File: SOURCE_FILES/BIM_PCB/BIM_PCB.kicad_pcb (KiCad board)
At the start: 4 copper layers, 58.5 x 72.5 mm, 195 parts, among them J1 Conn_02x09_Counter_Clockwise, J2 nano_sim, J3 Conn_01x06, J4 Micro_SD_Card, Q1 SSM3J328R-HXY, Q2 SSM3J328R-HXY, Q3 IRLML0100TRPBF, Q5 BSN20, Q6 BSN20, SW1 reset, U1 STM32F103C8Tx, U10 TBU-CA065-200-WH, U11 SSP3485U, U12 TBU-CA065-200-WH, U13 ATA6561-GAQW-N, U14 WAS3157B, U15 MC74HC4052A, U16 SY8089AAAC, U17 XC6206PxxxMR, U18 TBU-CA065-200-WH, U19 SSP3485U, U2 PCF8523TK, U20 TBU-CA065-200-WH, U3 A9G_MODULE, U4 TBU-CA065-200-WH, U5 SSP3485U, U6 TBU-CA065-200-WH, U7 WAS3157B, U8 W25Q32JVSS, U9 ATA6561-GAQW-N, Y1 8MHz, Y2 32.678KHz, Y3 32.678KHz

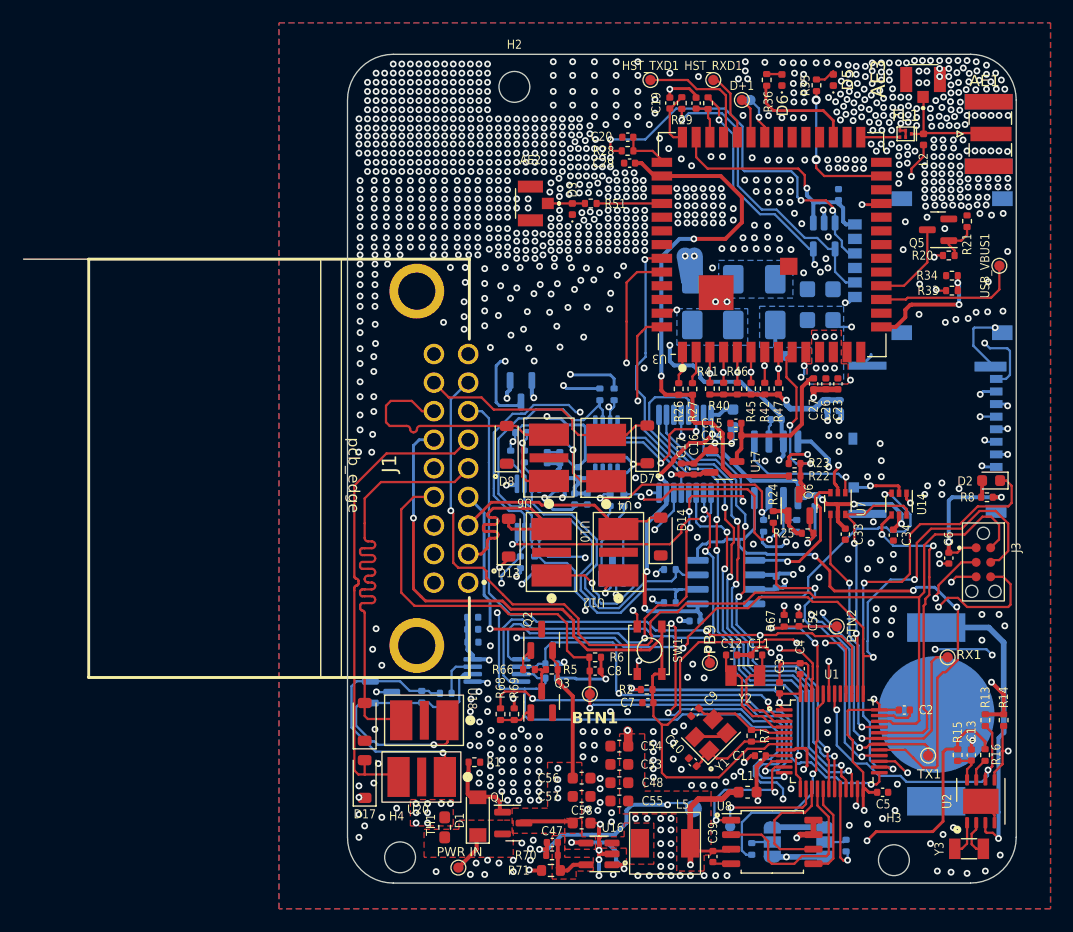
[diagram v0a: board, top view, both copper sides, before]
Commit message: all items updated
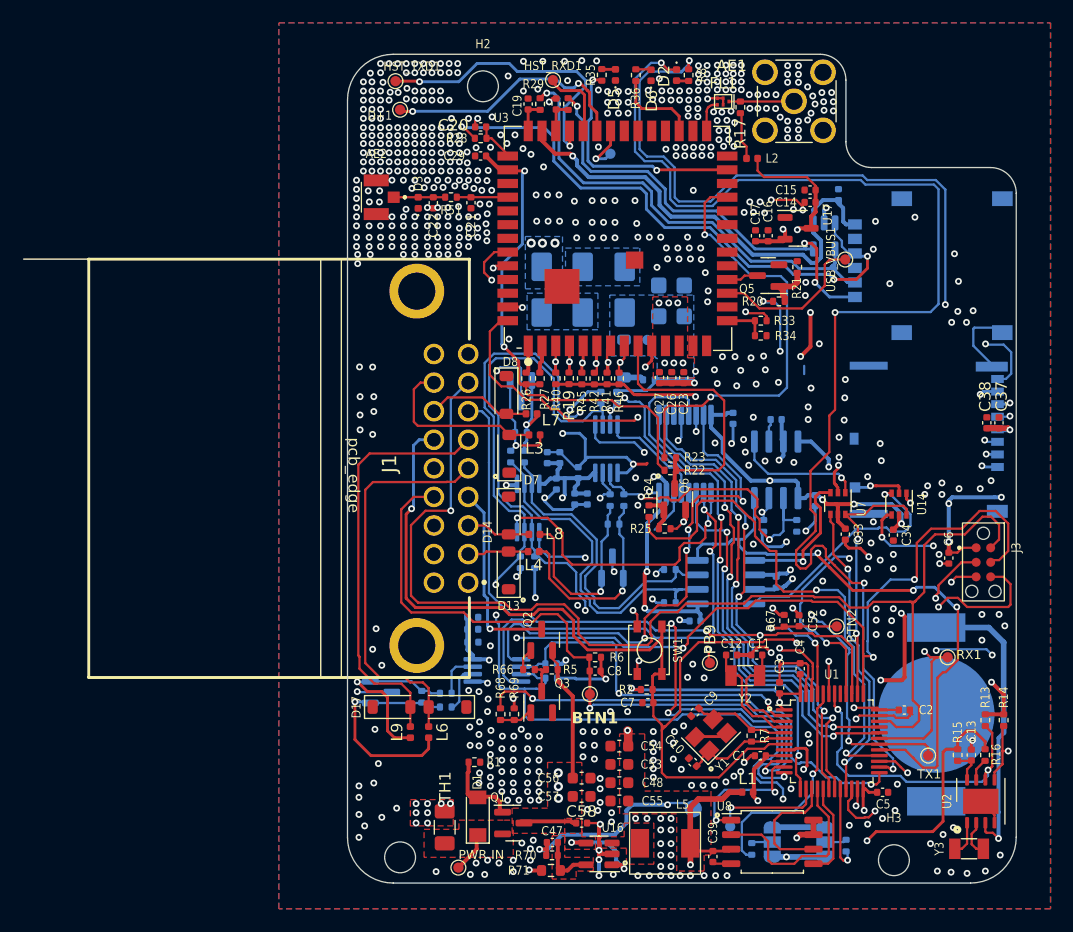
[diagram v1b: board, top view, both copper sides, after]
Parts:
- removed AE3: Antenna_Shield, greencharge-footprints:UFL_COAX_CONN23370191
- removed J4: Micro_SD_Card, MACHADA_footprints:MOLEX_503398-1892
- removed R47: 10k, Resistor_SMD:R_0402_1005Metric
- removed U10, U12, U18, U20, U4, U6: TBU-CA065-200-WH, MACHADA_footprints:TBU-CA065-200-WH
- added C37: 0.1u, Capacitor_SMD:C_0402_1005Metric, F.Cu at (93.0, 90.0)
- added C38: 1u, Capacitor_SMD:C_0402_1005Metric, F.Cu at (91.9, 90.0)
- added D19: 4.4-4.5 ZENER, Diode_SMD:D_SOD-123, B.Cu at (60.2, 84.4)
- added J7: Micro_SD_Card, MACHADA_footprints:MOLEX_503398-1892, B.Cu at (87.2, 91.5)
- added L3: ferrite bead, Inductor_SMD:L_0402_1005Metric, F.Cu at (52.4, 91.0)
- added L4: ferrite bead, Inductor_SMD:L_0402_1005Metric, F.Cu at (52.3, 101.2)
- added L6: ferrite bead, Inductor_SMD:L_0402_1005Metric, F.Cu at (43.1, 117.0)
- added L7: ferrite bead, Inductor_SMD:L_0402_1005Metric, F.Cu at (52.1, 89.2)
- added L8: ferrite bead, Inductor_SMD:L_0402_1005Metric, F.Cu at (52.4, 99.8)
- added L9: ferrite bead, Inductor_SMD:L_0402_1005Metric, F.Cu at (41.5, 117.0)
- added R17: 22R, Resistor_SMD:R_0402_1005Metric, F.Cu at (70.4, 62.4)
- added R18: 49.9R, Resistor_SMD:R_0402_1005Metric, B.Cu at (62.4, 86.2)
- added R19: 10k, Resistor_SMD:R_0402_1005Metric, F.Cu at (55.4, 86.1)
- AE1: footprint Connector_Coaxial:SMA_Samtec_SMA-J-P-X-ST-EM1_EdgeMount -> Connector_Coaxial:SMA_Molex_73251-2200_Horizontal
- C21: value 0.1u -> C_Small; moved to F.Cu
- C22: value 1u -> C_Small; moved to F.Cu
- C46, C58: footprint Capacitor_SMD:C_0603_1608Metric -> Capacitor_SMD:C_0402_1005Metric
- D10: value SS310 -> RS1K-E3/5ATSS310
- D2: footprint LED_SMD:LED_0603_1608Metric -> LED_SMD:LED_0402_1005Metric
- H4: moved to B.Cu
- L1: footprint Inductor_SMD:L_0603_1608Metric -> Inductor_SMD:L_0402_1005Metric
- Q5, Q6: value BSN20 -> IRLML0100TRPBF
- TH1: footprint Fuse:Fuse_0603_1608Metric_Pad1.05x0.95mm_HandSolder -> Fuse:Fuse_1206_3216Metric
- moved R8 45.2 mm to (65.8, 59.6), turned to -90 degrees
- moved D2 44.9 mm to (64.8, 59.6), turned to -90 degrees
- moved C22 39.7 mm to (43.5, 70.7), turned to 90 degrees
- moved C21 35.9 mm to (46.8, 70.7), turned to 90 degrees
- moved D+1 29.9 mm to (40.6, 62.6)
- moved HST_TXD1 22.3 mm to (40.2, 60.1)
- moved C15 21.4 mm to (76.5, 69.6)
- moved C16 21.4 mm to (72.8, 73.6)
- moved C17 21.4 mm to (71.7, 73.6)
- moved C14 21.4 mm to (76.5, 70.7)
- moved U17 21.4 mm to (75.4, 73.0)
- moved D5 19.1 mm to (59.4, 59.6)
- moved R35 18.8 mm to (58.2, 59.6)
- moved R34 17.5 mm to (72.2, 82.4), turned to 180 degrees
- moved AE1 17.3 mm to (75.1, 61.9), turned to -90 degrees
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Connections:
- C21 pad 1: 2V8 -> GND
- C21 pad 2: GND -> Net-(U3-GSM_RF)
- C22 pad 1: 2V8 -> GND
- C22 pad 2: GND -> Net-(AE2-A)
- L2 pad 1: Net-(AE1-A) -> Net-(L2-Pad1)
- R40 pad 2: /A9G_GSM_GPRS_MODULE/TF_CARD_CONN/SD_D2 -> /A9G_GSM_GPRS_MODULE/TF_CARD_CONN/SD_D3
- R41 pad 2: /A9G_GSM_GPRS_MODULE/TF_CARD_CONN/SD_D3 -> /A9G_GSM_GPRS_MODULE/TF_CARD_CONN/SD_CMD
- R42 pad 2: /A9G_GSM_GPRS_MODULE/TF_CARD_CONN/SD_CMD -> /A9G_GSM_GPRS_MODULE/TF_CARD_CONN/SD_D0
- R45 pad 2: /A9G_GSM_GPRS_MODULE/TF_CARD_CONN/SD_D0 -> /A9G_GSM_GPRS_MODULE/TF_CARD_CONN/SD_D1
- R46 pad 2: /A9G_GSM_GPRS_MODULE/TF_CARD_CONN/SD_D1 -> /A9G_GSM_GPRS_MODULE/TF_CARD_CONN/SD_CLK
- U1 pad 12: /A9G_GSM_GPRS_MODULE/GPS_TXD -> /A9G_GSM_GPRS_MODULE/GPS_RXD
- U1 pad 13: /A9G_GSM_GPRS_MODULE/GPS_RXD -> /A9G_GSM_GPRS_MODULE/GPS_TXD
- U1 pad 21: /STM32FC8T6_MCU/RS485_RO -> /MULTIPLEXER_SWITCH_WAS3157B-6/SIG1_IN
- U1 pad 22: /STM32FC8T6_MCU/RS485_DI -> /MULTIPLEXER_SWITCH_WAS3157B-6/SIG2_IN
- U1 pad 32: /MULTIPLEXER_SWITCH_WAS3157B-6/SIG2_IN -> /STM32FC8T6_MCU/RS485_DI
- U1 pad 33: /MULTIPLEXER_SWITCH_WAS3157B-6/SIG1_IN -> /STM32FC8T6_MCU/RS485_RO
- U3 pad 49: /A9G_GSM_GPRS_MODULE/GPS_RXD -> /A9G_GSM_GPRS_MODULE/GPS_TXD
- U3 pad 50: /A9G_GSM_GPRS_MODULE/GPS_TXD -> /A9G_GSM_GPRS_MODULE/GPS_RXD
- U3 pad 53: /STM32FC8T6_MCU/RX1 -> /STM32FC8T6_MCU/TX1
- U3 pad 54: /STM32FC8T6_MCU/TX1 -> /STM32FC8T6_MCU/RX1
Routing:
- net /STM32FC8T6_MCU/3v3_stm: track 113.6 -> 191.5 mm, vias 9 -> 14
- net Net-(D2-K): track 39.9 -> 113.4 mm, vias 2 -> 4
- net /A9G_GSM_GPRS_MODULE/Sim_Restart: track 67.7 -> 46.6 mm, vias 2 -> 4
- net /MULTIPLEXER_SWITCH_WAS3157B-6/SIG2_IN: track 27.8 -> 48.6 mm, vias 2 -> 3
- net /A9G_GSM_GPRS_MODULE/V_Sim: track 22.5 -> 41.5 mm
- net Net-(U3-USB_P): track 3.58 -> 22.2 mm, vias 0 -> 2
- net /A9G_GSM_GPRS_MODULE/GPS_RXD: track 57.5 -> 75.3 mm
- net /A9G_GSM_GPRS_MODULE/PWRKEY: track 28.4 -> 45.6 mm
- net /A9G_GSM_GPRS_MODULE/IO29: track 55.6 -> 38.8 mm
- net Net-(J2-RST): track 34.4 -> 51.0 mm
- net 4.2V_SIMPWR: track 46.7 -> 30.7 mm, vias 9 -> 8
- net /A9G_GSM_GPRS_MODULE/TF_CARD_CONN/SD_D0: track 28.7 -> 44.3 mm
- net Net-(J2-CLK): track 26.6 -> 41.7 mm
- net Net-(U3-HST_RXD): track 10.9 -> 26.0 mm, vias 0 -> 2
- net 2V8: track 62.8 -> 77.8 mm, vias 3 -> 5
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- added copper zone on B.Cu, net +5V
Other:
- outline, holes or cut-outs redrawn
